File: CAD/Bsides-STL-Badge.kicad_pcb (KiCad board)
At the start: 2 copper layers, 93.5 x 137.1 mm, 7 parts

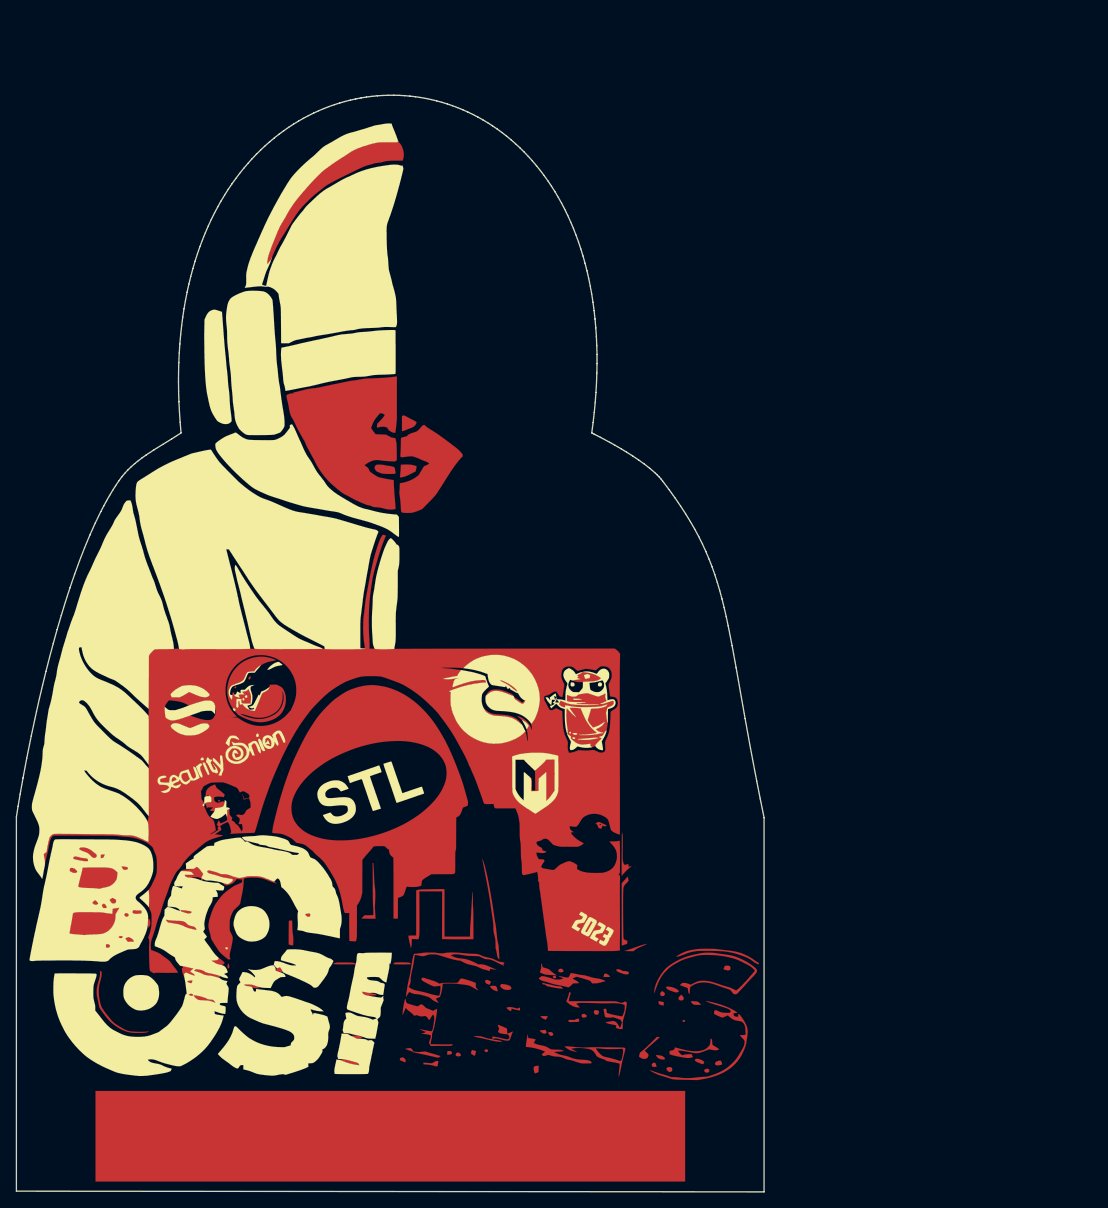
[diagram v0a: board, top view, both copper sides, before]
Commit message: laying out with no elect
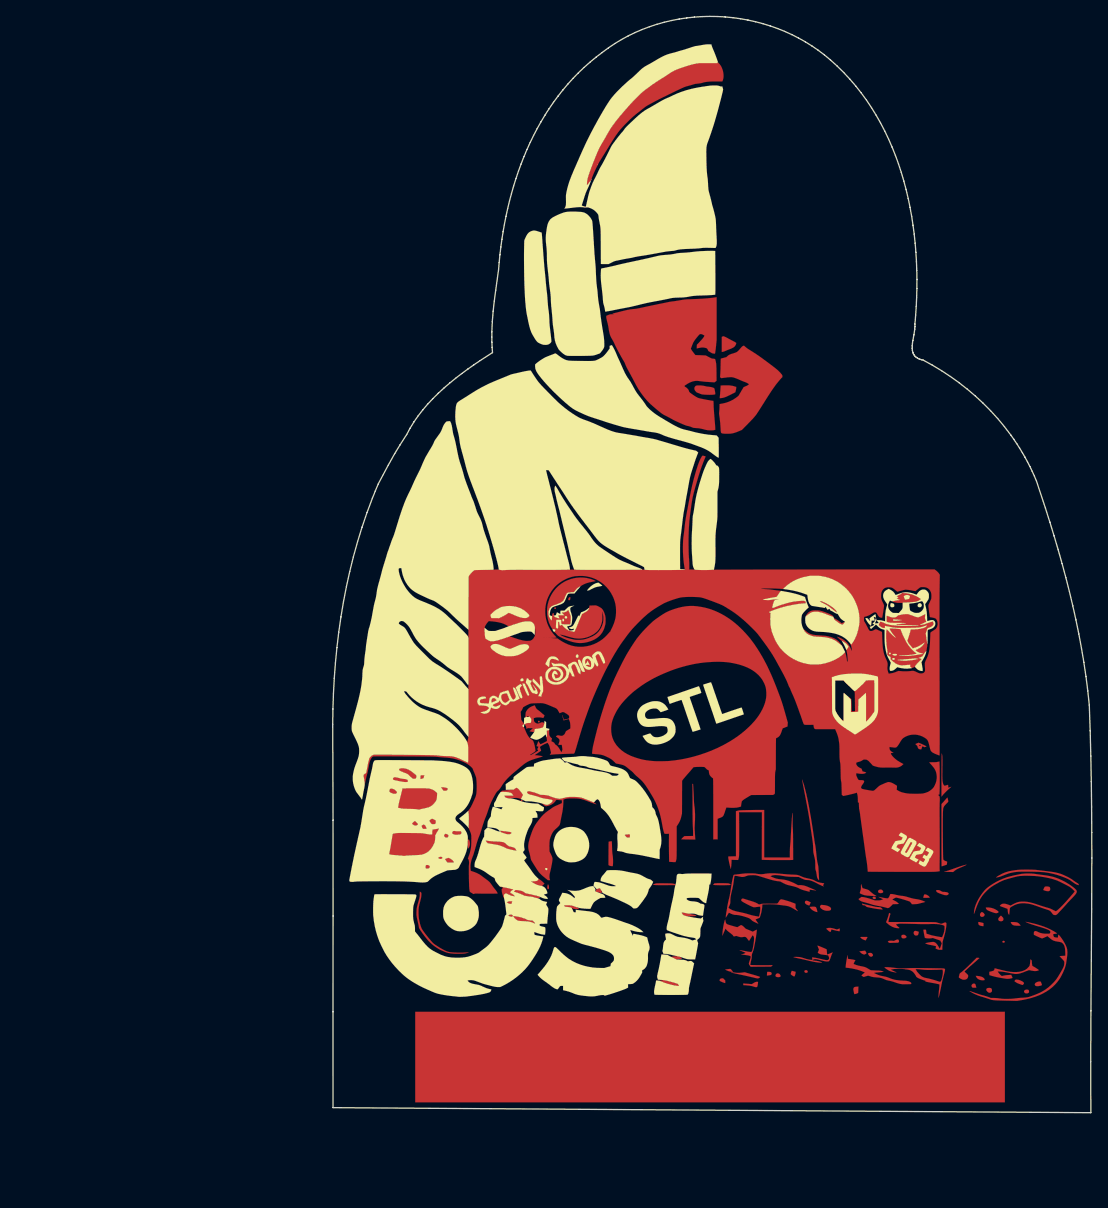
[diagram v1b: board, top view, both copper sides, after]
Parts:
- removed the G*** at (88.9, 104.5) (x7)
- added G*** (x7): LOGO, LOGO, F.Cu at (128.8, 94.6)
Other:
- board size 93.5 x 137.1 mm -> 94.9 x 137 mm
